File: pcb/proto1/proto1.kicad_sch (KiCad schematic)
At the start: 158 parts, among them J1 AudioJack3, J2 AudioJack3, J3 AUX, J4 LEFT, J5 RIGHT, SW1 SW_StartPause, SW2 SW_Stop, SW3 SW_Reverse, SW4 SW_Restart, SW5 SW_LoopIn, SW6 SW_LoopOut, SW7 SW_LoopInc, SW8 SW_LoopDec, U1 ATSAM4C4, U10 SAM-JTAG-10, U11 SAM-JTAG-10, U12 NE5532, U13 NE5532, U14 SAM-JTAG-10, U2 NDS36P, U3 ATSAMD21E17D-A, U4 ATSAMD21E17D-A, U5 NE5532, U6 PCM1742, U7 NE5532, U8 PCM1807, U9 NE5532, Y1 Crystal, Y2 Crystal, Y3 20MHz

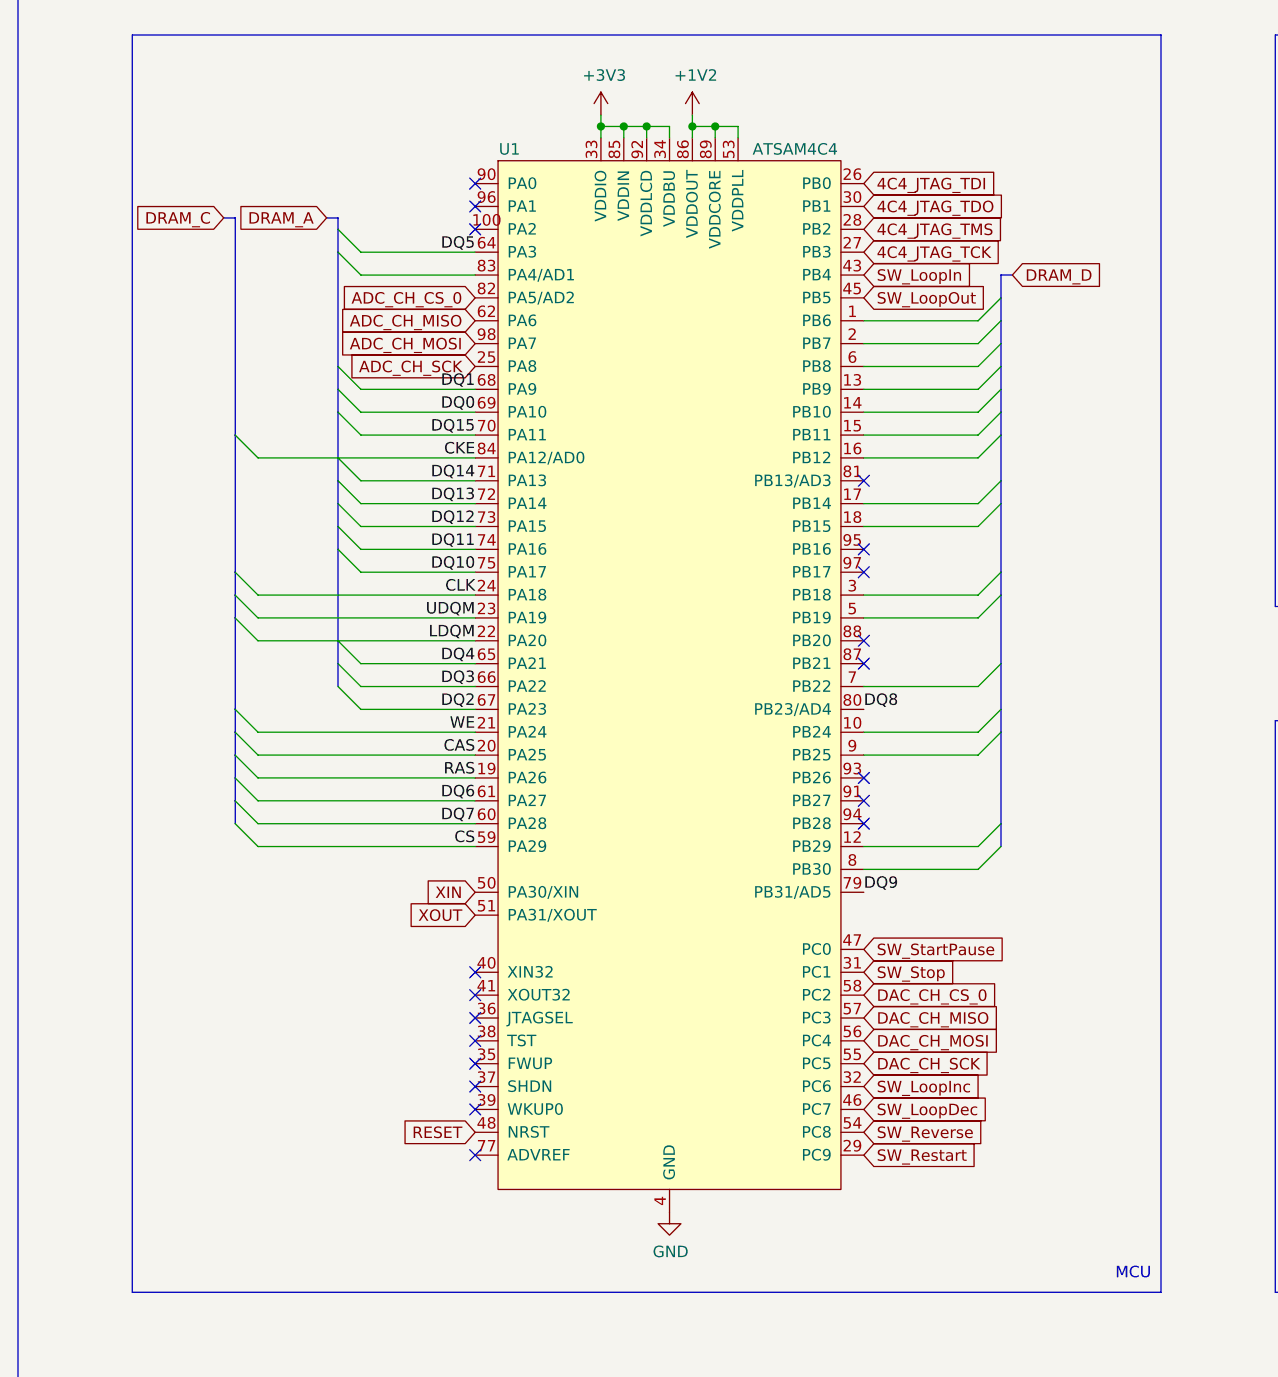
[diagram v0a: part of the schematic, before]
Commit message: .
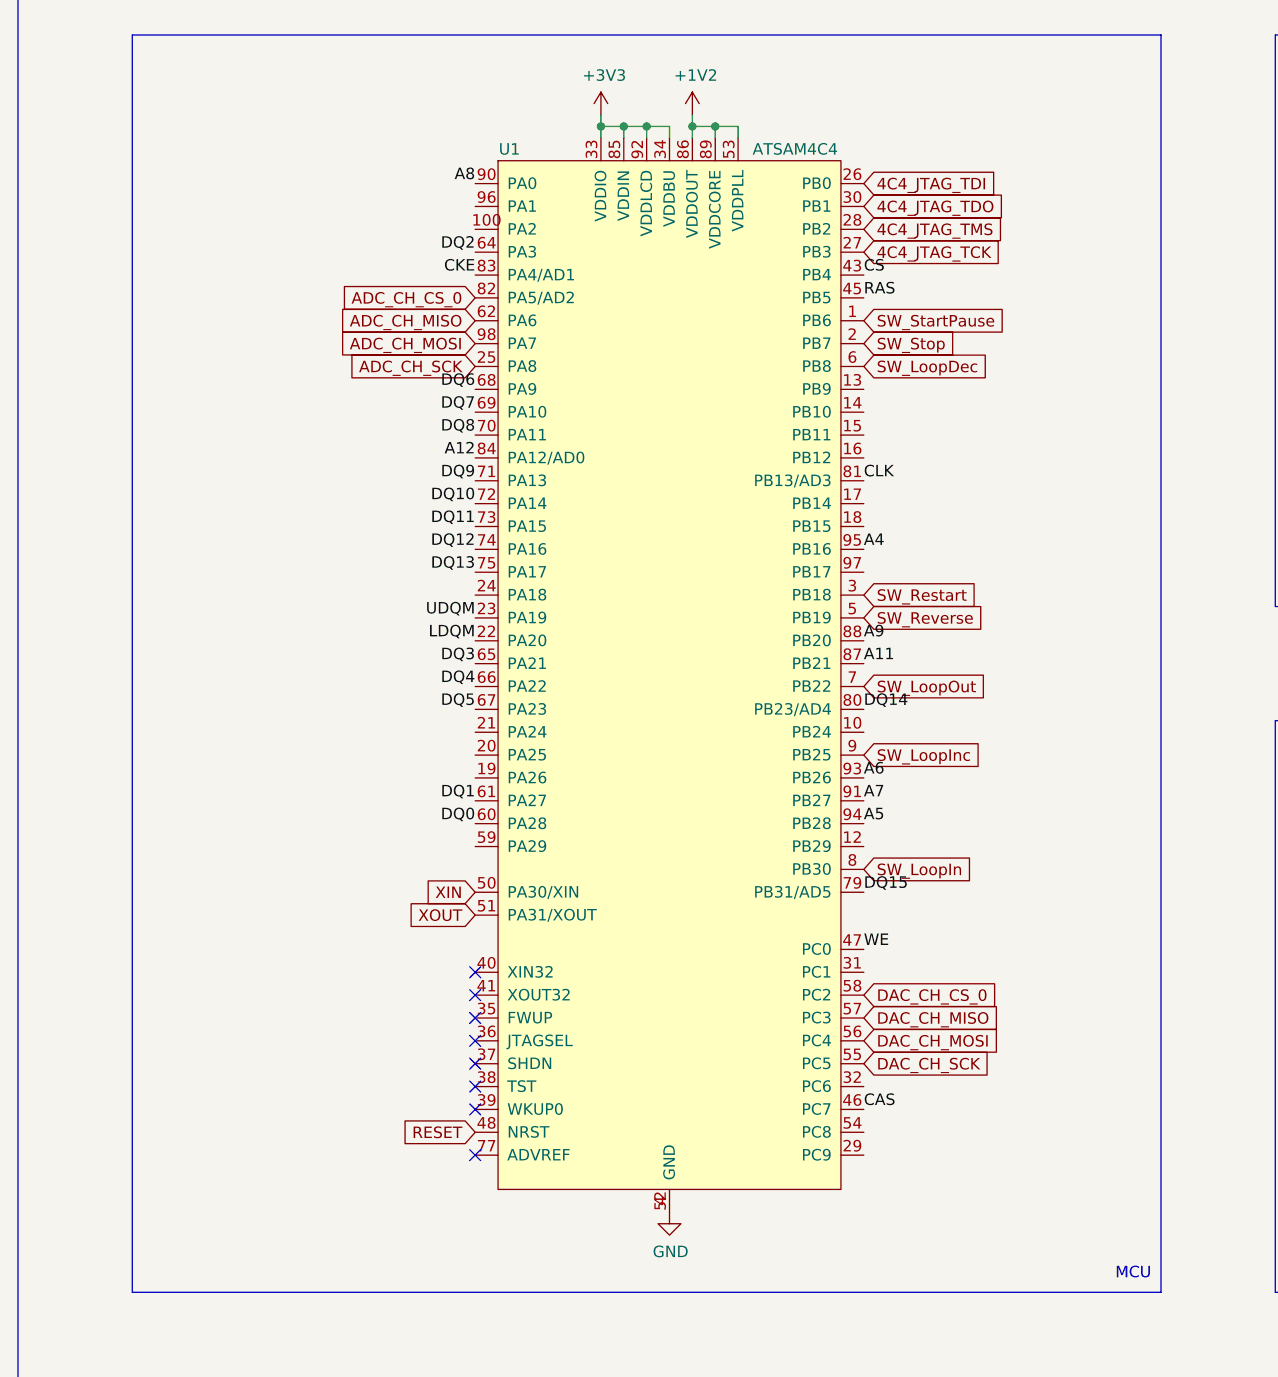
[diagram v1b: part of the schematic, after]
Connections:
- net A11: now also U1.87 (PB21)
- net A12: now also U1.84 (PA12/AD0)
- net A4: now also U1.95 (PB16)
- net A5: now also U1.94 (PB28)
- net A6: now also U1.93 (PB26)
- net A7: now also U1.91 (PB27)
- net A8: now also U1.90 (PA0)
- net A9: now also U1.88 (PB20)
- net CAS: now also U1.46 (PC7); no longer U1.20 (PA25)
- net CKE: now also U1.83 (PA4/AD1); no longer U1.84 (PA12/AD0)
- net CLK: now also U1.81 (PB13/AD3); no longer U1.24 (PA18)
- net CS: now also U1.43 (PB4); no longer U1.59 (PA29)
- net DQ0: now also U1.60 (PA28); no longer U1.69 (PA10)
- net DQ1: now also U1.61 (PA27); no longer U1.68 (PA9)
- net DQ10: now also U1.72 (PA14); no longer U1.75 (PA17)
- net DQ11: now also U1.73 (PA15); no longer U1.74 (PA16)
- net DQ12: now also U1.74 (PA16); no longer U1.73 (PA15)
- net DQ13: now also U1.75 (PA17); no longer U1.72 (PA14)
- net DQ14: now also U1.80 (PB23/AD4); no longer U1.71 (PA13)
- net DQ15: now also U1.79 (PB31/AD5); no longer U1.70 (PA11)
- net DQ2: now also U1.64 (PA3); no longer U1.67 (PA23)
- net DQ3: now also U1.65 (PA21); no longer U1.66 (PA22)
- net DQ4: now also U1.66 (PA22); no longer U1.65 (PA21)
- net DQ5: now also U1.67 (PA23); no longer U1.64 (PA3)
- net DQ6: now also U1.68 (PA9); no longer U1.61 (PA27)
- net DQ7: now also U1.69 (PA10); no longer U1.60 (PA28)
- net DQ8: now also U1.70 (PA11); no longer U1.80 (PB23/AD4)
- net DQ9: now also U1.71 (PA13); no longer U1.79 (PB31/AD5)
- net GND: now also U1.52 (GND)
- net RAS: now also U1.45 (PB5); no longer U1.19 (PA26)
- net SW_LoopDec: now also U1.6 (PB8); no longer U1.46 (PC7)
- net SW_LoopIn: now also U1.8 (PB30); no longer U1.43 (PB4)
- net SW_LoopInc: now also U1.9 (PB25); no longer U1.32 (PC6)
- net SW_LoopOut: now also U1.7 (PB22); no longer U1.45 (PB5)
- net SW_Restart: now also U1.3 (PB18); no longer U1.29 (PC9)
- net SW_Reverse: now also U1.5 (PB19); no longer U1.54 (PC8)
- net SW_StartPause: now also U1.1 (PB6); no longer U1.47 (PC0)
- net SW_Stop: now also U1.2 (PB7); no longer U1.31 (PC1)
- net WE: now also U1.47 (PC0); no longer U1.21 (PA24)
- no-connect marks 47 -> 36
